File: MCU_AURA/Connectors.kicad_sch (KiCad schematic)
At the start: 10 parts, among them J400 532617004, J401 532617004, J402 532617004, J403 532617010, J404 532617007, J405 532617007, J406 532617012, J407 532614005

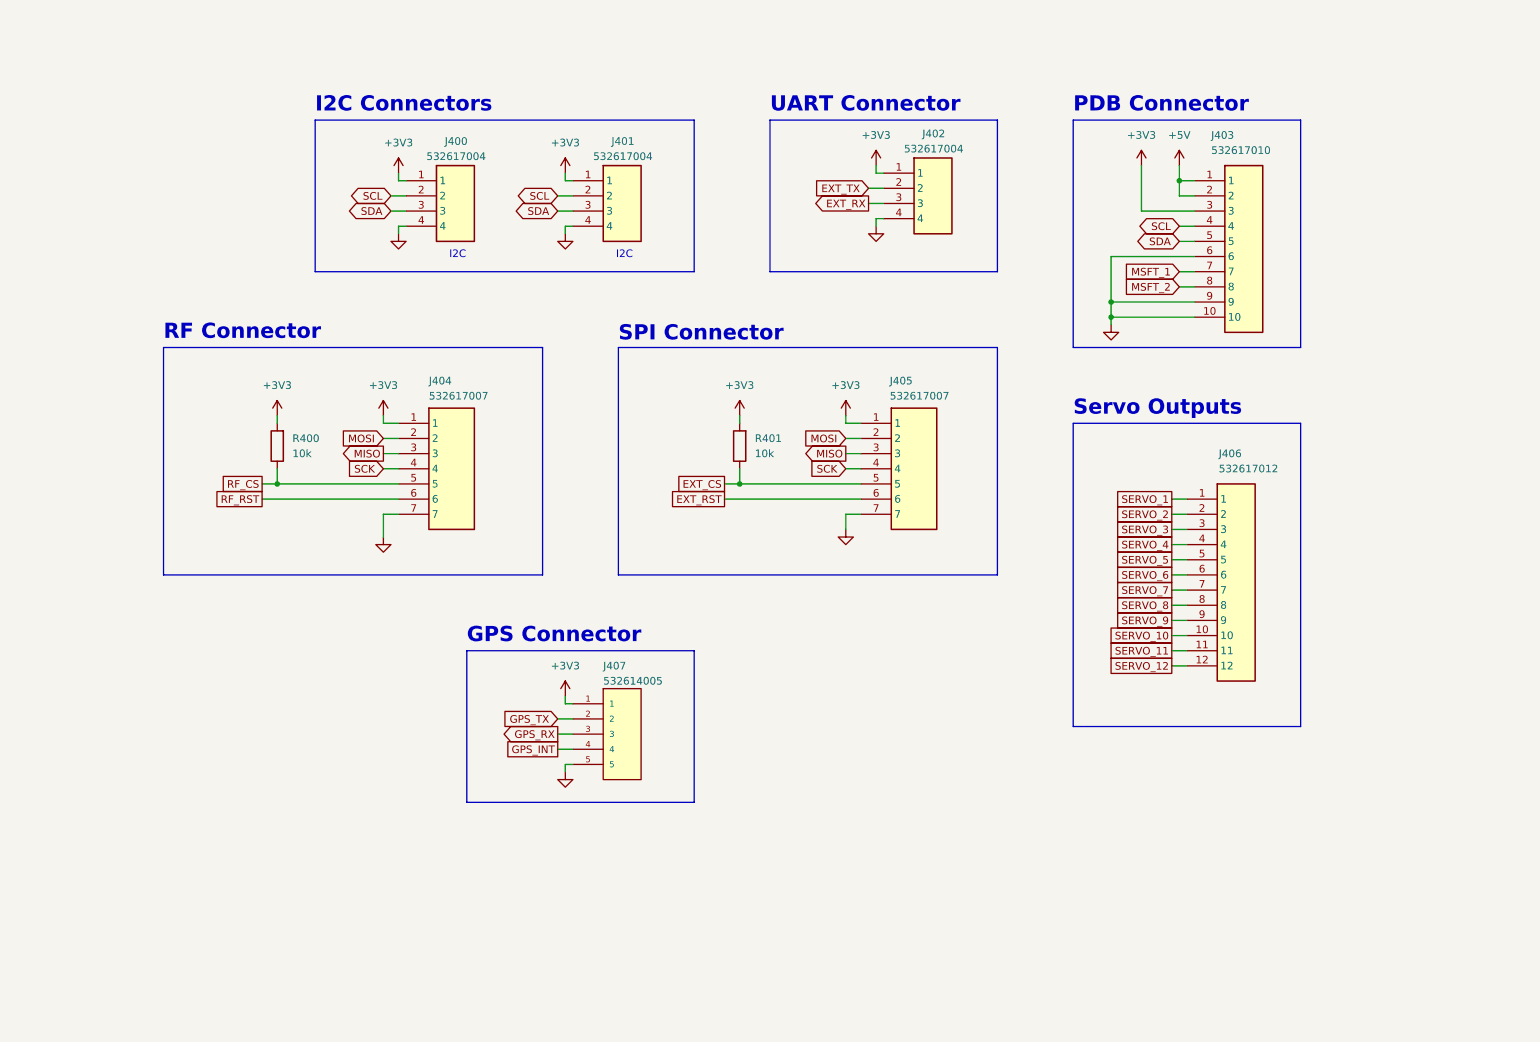
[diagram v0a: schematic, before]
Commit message: Started Routing
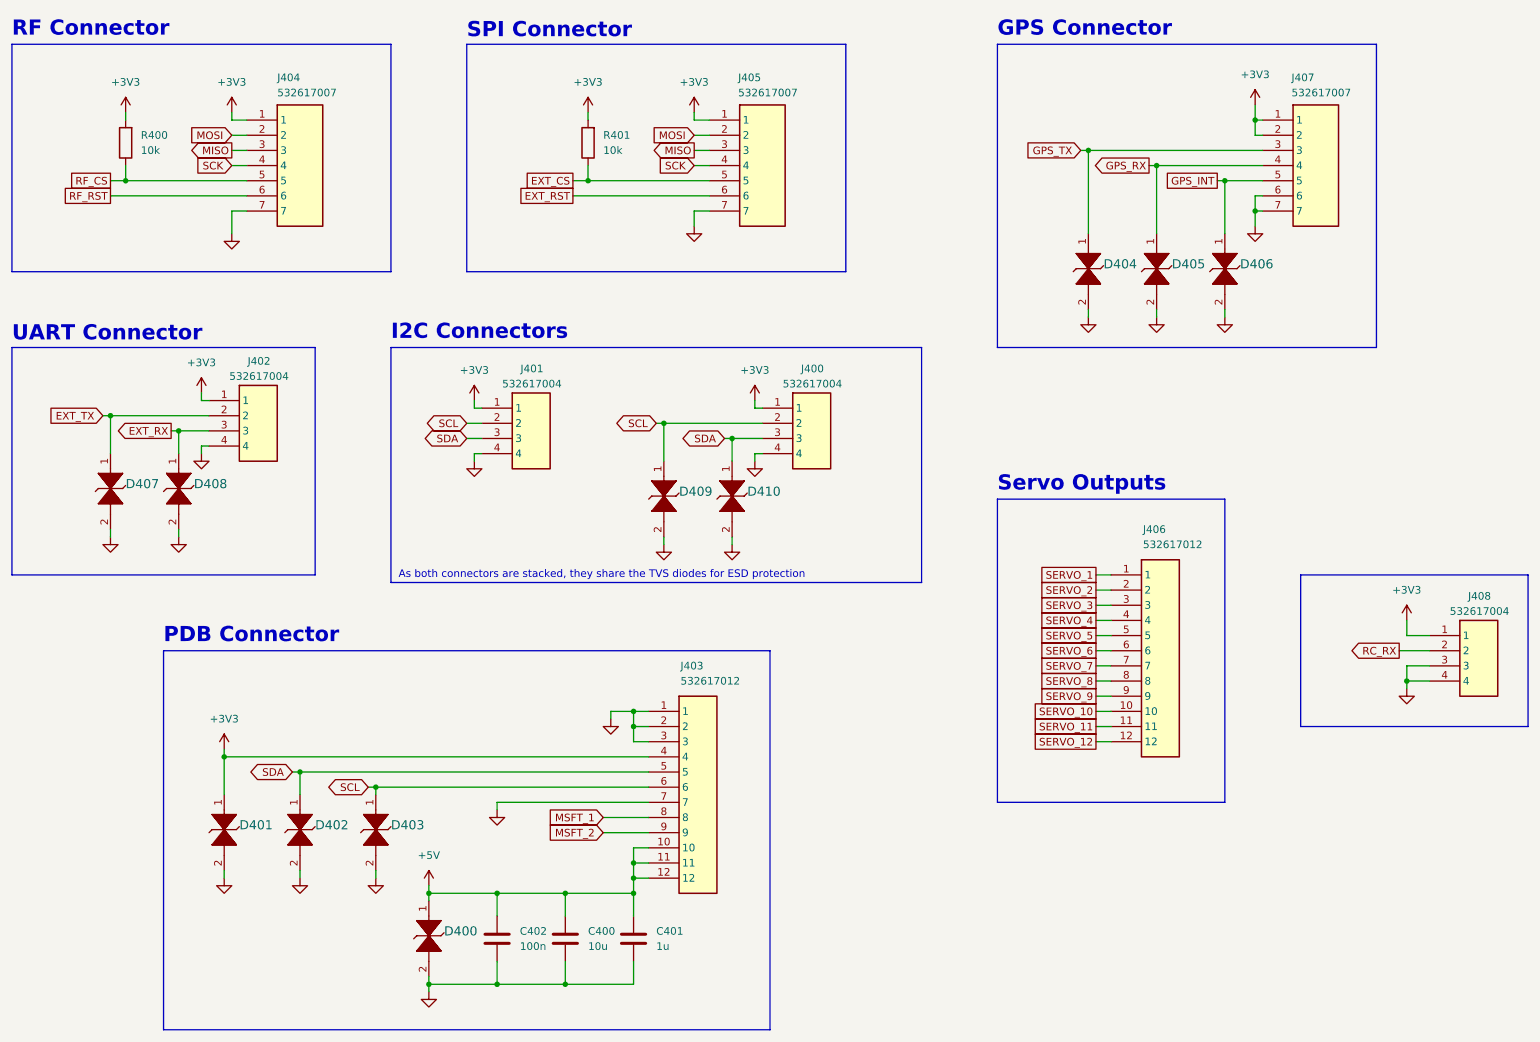
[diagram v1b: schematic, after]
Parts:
- removed J403: 532617010, 532617010:532617010, symbol 532617010:532617010
- removed J407: 532614005, 532614005:CONN_532610000-SD_05_MOL, symbol 532614005:532614005
- added C400: 10u, Capacitor_SMD:C_0402_1005Metric, symbol Device:C
- added C401: 1u, Capacitor_SMD:C_0402_1005Metric, symbol Device:C
- added C402: 100n, Capacitor_SMD:C_0402_1005Metric, symbol Device:C
- added D400, D401, D402, D403, D404, D405, D406, D407, D408, D409, D410: TPD1E05U06DPYR, TPD1E05U06DPYR:DIO_TPD1E05U06DPYR, symbol ESDALC5_1BM2:ESDALC5-1BM2
- added J403: 532617012, 532611271:53261-1271, symbol 532617012:532617012
- added J407: 532617007, 532610771:532610771, symbol 532617007:532617007
- added J408: 532617004, 532610471:53261-0471, symbol 532617004:532617004
- J400, J401, J402: footprint 532617004:532617004 -> 532610471:53261-0471
- J404, J405: footprint 532617007:532617007 -> 532610771:532610771
- J406: footprint 532617012:532617012 -> 532611271:53261-1271
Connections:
- net +3V3: now also D401.1, J403.4, J407.1, J407.2, J408.1
- net +5V: now also C400.1, C401.1, C402.1, D400.1, J403.10, J403.11, J403.12
- net EXT_RX: now also D408.1
- net EXT_TX: now also D407.1
- net GND: now also C400.2, C401.2, C402.2, D400.2, D401.2, D402.2, D403.2, D404.2, D405.2, D406.2, D407.2, D408.2, D409.2, D410.2, J403.1, J403.2, J403.3, J403.7, J407.6, J407.7, J408.3, J408.4
- net GPS_INT: now also D406.1, J407.5
- net GPS_RX: now also D405.1, J407.4
- net GPS_TX: now also D404.1, J407.3
- net MSFT_1: now also J403.8
- net MSFT_2: now also J403.9
- net SCL: now also D403.1, D409.1, J403.6
- net SDA: now also D402.1, D410.1, J403.5
- new net RC_RX: J408.2
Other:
- note added: "As both connectors are stacked, they share the TVS diodes for ESD protection"
- note removed: "I2C"
- moved on the sheet: J400, J402, J404, J405, J406, R400, R401

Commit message: Second Iteration MCU
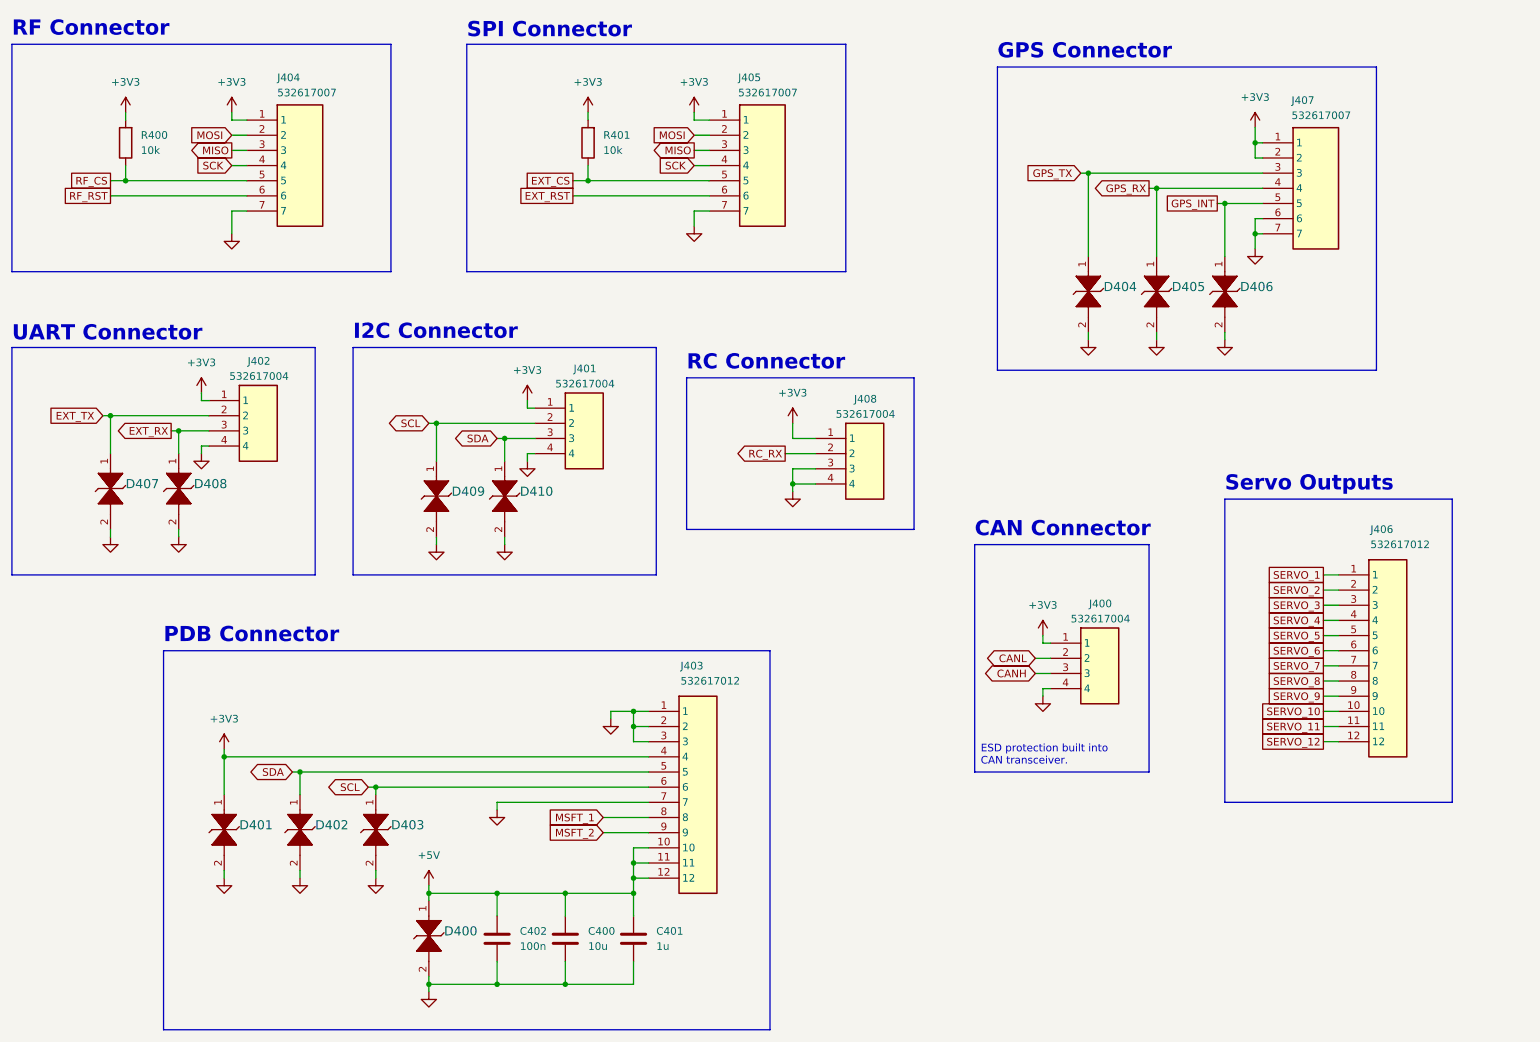
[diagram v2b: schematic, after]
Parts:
- renumbered J401 to J400, J400 to J401
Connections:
- net SCL: no longer J400.2
- net SDA: no longer J400.3
- new net CANH: J400.3
- new net CANL: J400.2
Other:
- note added: "CAN Connector"
- note added: "ESD protection built into CAN transceiver."
- note added: "I2C Connector"
- note added: "RC Connector"
- note removed: "As both connectors are stacked, they share the TVS diodes for ESD protection"
- note removed: "I2C Connectors"
- moved on the sheet: D404, D405, D406, D409, D410, J400, J401, J406, J407, J408
